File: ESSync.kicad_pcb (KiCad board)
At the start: 2 copper layers, 82.5 x 56.5 mm, 9 parts, among them SW1 SW_Slide_DPDT, U3 ESP32-C3-DevKitM-1

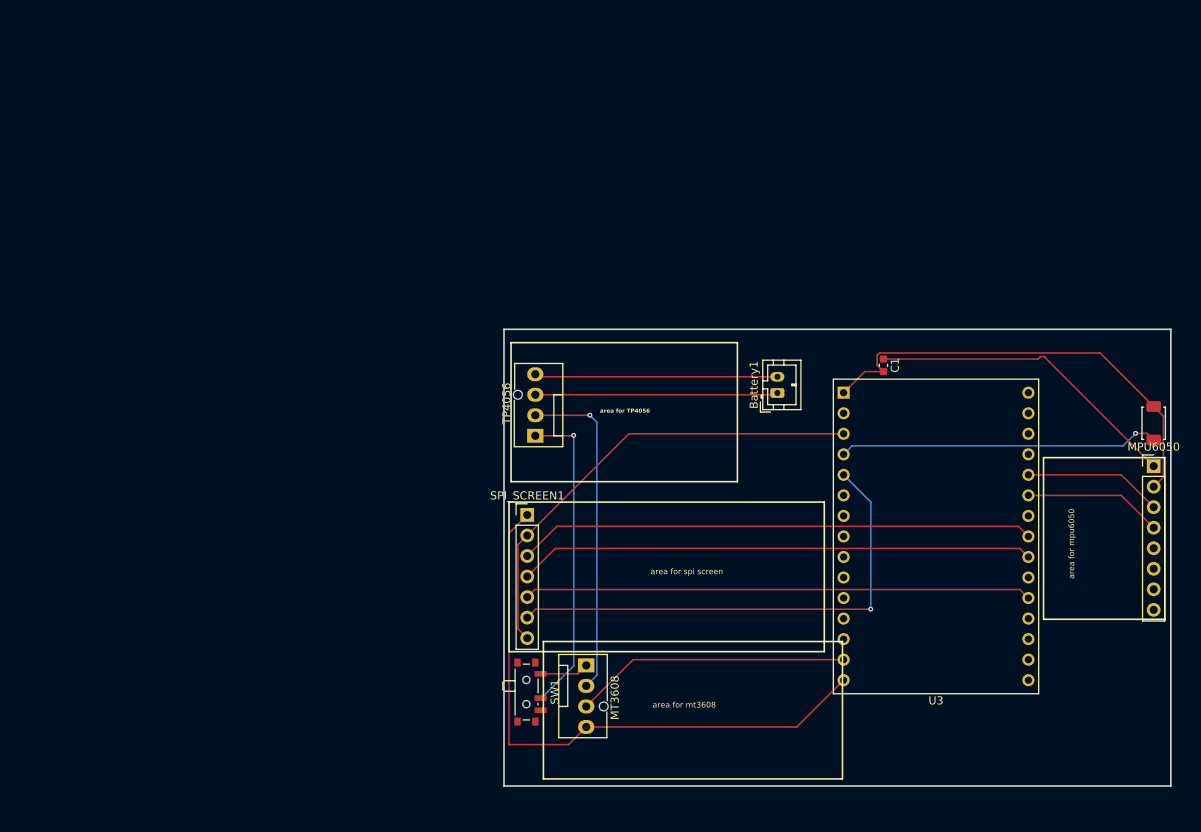
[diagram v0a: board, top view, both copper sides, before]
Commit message: Added updated files of pcb
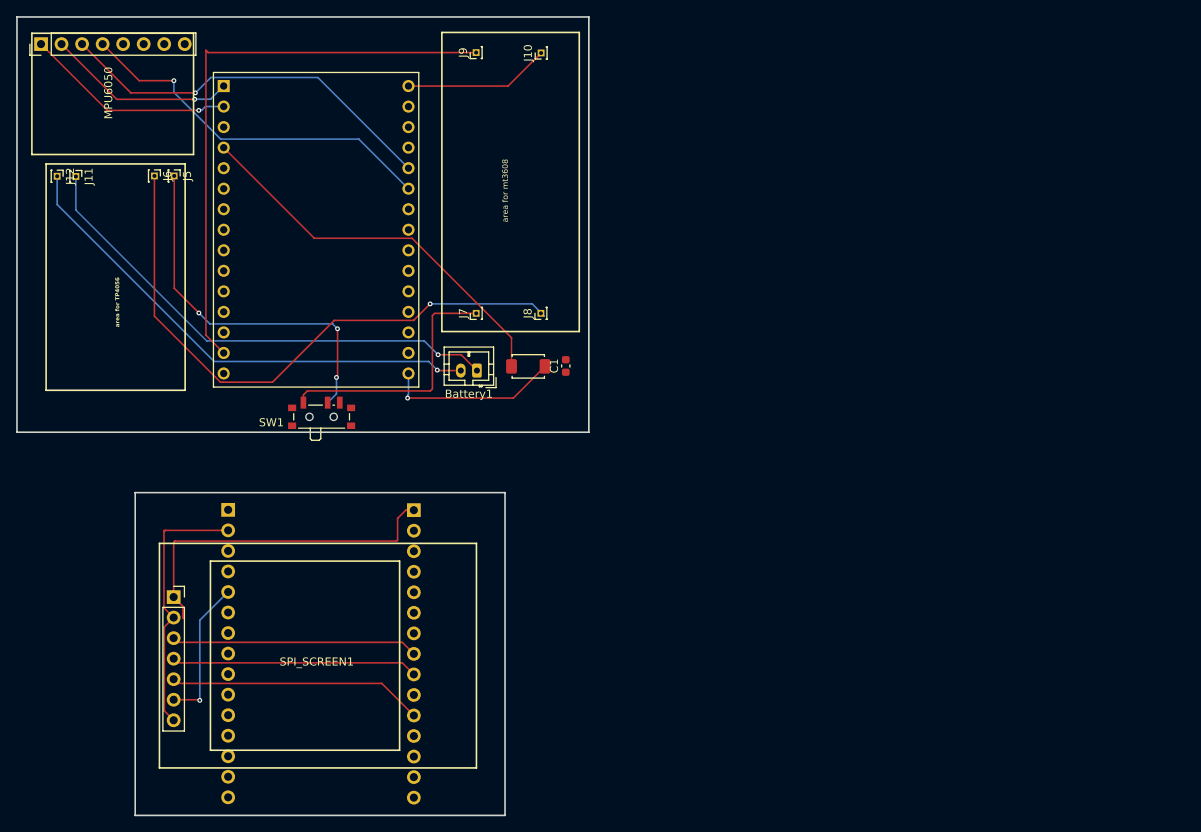
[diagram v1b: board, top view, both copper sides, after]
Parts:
- removed MT3608, TP4056: Conn_01x04, Connector:FanPinHeader_1x04_P2.54mm_Vertical
- added J1: Conn_01x15, Connector_PinSocket_2.54mm:PinSocket_1x15_P2.54mm_Vertical, B.Cu at (112.2, 103.5)
- added J10: Conn_01x01, Connector_PinHeader_1.00mm:PinHeader_1x01_P1.00mm_Vertical, F.Cu at (128.0, 46.9)
- added J11: Conn_01x01, Connector_PinHeader_1.00mm:PinHeader_1x01_P1.00mm_Vertical, F.Cu at (70.4, 62.2)
- added J12: Conn_01x01, Connector_PinHeader_1.00mm:PinHeader_1x01_P1.00mm_Vertical, F.Cu at (68.1, 62.2)
- added J2: Conn_01x15, Connector_PinSocket_2.54mm:PinSocket_1x15_P2.54mm_Vertical, B.Cu at (89.2, 103.5)
- added J5: Conn_01x01, Connector_PinHeader_1.00mm:PinHeader_1x01_P1.00mm_Vertical, F.Cu at (82.6, 62.1)
- added J6: Conn_01x01, Connector_PinHeader_1.00mm:PinHeader_1x01_P1.00mm_Vertical, F.Cu at (80.1, 62.1)
- added J7: Conn_01x01, Connector_PinHeader_1.00mm:PinHeader_1x01_P1.00mm_Vertical, F.Cu at (119.9, 79.2)
- added J8: Conn_01x01, Connector_PinHeader_1.00mm:PinHeader_1x01_P1.00mm_Vertical, F.Cu at (127.9, 79.2)
- added J9: Conn_01x01, Connector_PinHeader_1.00mm:PinHeader_1x01_P1.00mm_Vertical, F.Cu at (119.9, 46.9)
- SPI_SCREEN1: footprint Connector_PinHeader_2.54mm:PinHeader_1x07_P2.54mm_Vertical -> Connector_PinSocket_2.54mm:PinSocket_1x07_P2.54mm_Vertical
- moved MPU6050 147.2 mm to (66.1, 45.8), turned to 90 degrees
- moved U3 85.6 mm to (88.7, 51.0)
- moved S1 77.7 mm to (126.4, 85.7), turned to 0 degrees
- moved SPI_SCREEN1 44.9 mm to (82.5, 114.2)
- moved SW1 42.9 mm to (100.8, 91.6), turned to 0 degrees
- moved C1 39.3 mm to (131.0, 85.7), turned to 90 degrees
- moved Battery1 37.3 mm to (120.0, 86.2), turned to 180 degrees
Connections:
- U3 pad 20: /RES -> unconnected-(U3-IO4-Pad20)
- U3 pad 22: /SDA_SPI -> unconnected-(U3-IO6-Pad22)
- U3 pad 23: /SCL_SPI -> unconnected-(U3-IO7-Pad23)
- U3 pad 5: /DC -> unconnected-(U3-IO3-Pad5)
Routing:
- net /DC: track 60.9 -> 18.1 mm
- net +3.3V: track 97.2 -> 59.1 mm, vias 0 -> 1
- net +5V: track 34.2 -> 71.9 mm
- net /SCL_SPI: track 64.0 -> 30.5 mm
- net /SDA_SPI: track 63.9 -> 30.5 mm
- net /IN-: track 41.1 -> 73.6 mm
- net /BAT+: track 30.0 -> 62.0 mm, vias 0 -> 1
- net /BAT-: track 30.1 -> 61.9 mm, vias 0 -> 1
- net /RES: track 62.8 -> 31.6 mm
- net /SCL: track 17.2 -> 48.3 mm, vias 0 -> 1
- net /SDA: track 17.2 -> 46.1 mm, vias 0 -> 1
- net /IN+: track 6.08 -> 31.8 mm
- net GND: track 130.4 -> 106.2 mm, vias 0 -> 2
- net /GPIO2: track 39.8 -> 48.9 mm, vias 1 -> 0
- net /OUT+: track 38.9 -> 46.0 mm, vias 1 -> 3
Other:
- board size 82.5 x 56.5 mm -> 70.8 x 98.8 mm
- board text removed: "area for mpu6050"
- board text removed: "area for spi screen"
